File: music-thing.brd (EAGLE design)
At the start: 177.5 x 129.5 mm, 6 parts

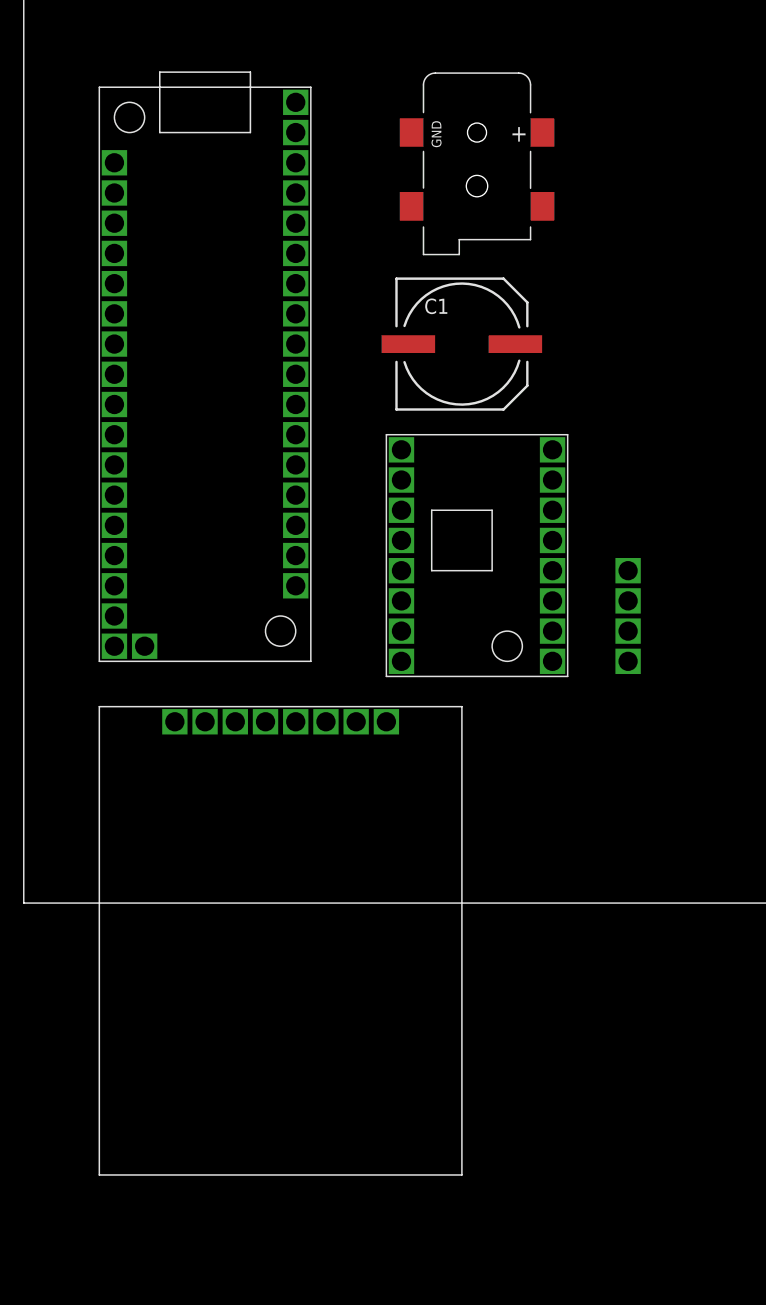
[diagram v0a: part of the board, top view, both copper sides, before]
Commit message: finalize
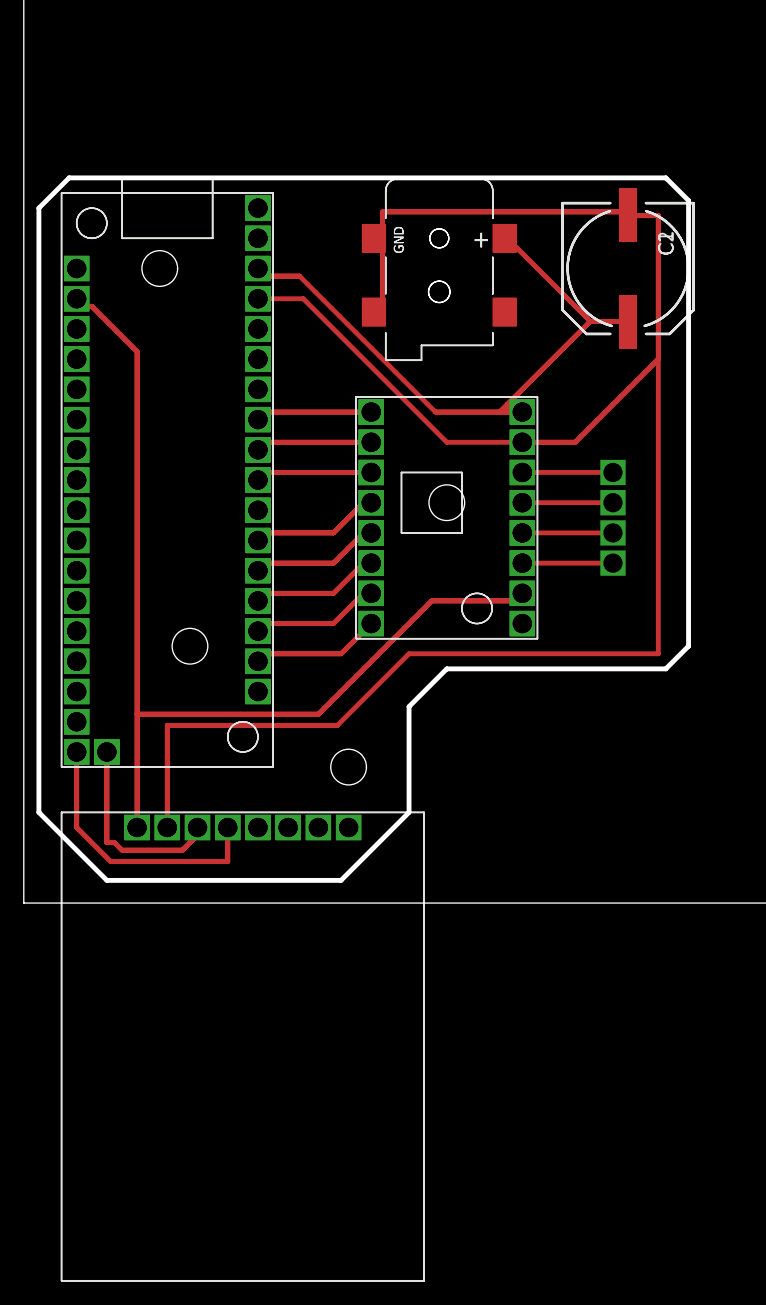
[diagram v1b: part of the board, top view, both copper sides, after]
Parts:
- added C2: 100uF, SparkFun-Capacitors:NIC_10X10.5_CAP
- added CN2: (no value), adafruit:DCJACK_2MM_SMT
- added E$1: (no value), weller-eagle:CON-MOTOR
- added U$5: ASTAR32U4MINI, weller-eagle:ASTAR32U4MINI
- added U$6: CON-USB-READER-V18, weller-eagle:CON-USB-READER-V18
- U$4: value CON-MOTOR -> A4998; device weller-eagle:CON-MOTOR -> weller-eagle:A4998
- moved U$4 20.4 mm to (27.9, 22.2)
- moved C1 15.3 mm to (50.8, 53.3), turned to 270 degrees
- moved U$2 9.44 mm to (3.17, 11.4)
- moved U$3 9.44 mm to (33.7, -31.8)
- moved CN1 9.44 mm to (34.9, 55.9)
- moved U$1 4.07 mm to (27.9, 22.2)
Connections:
- removed net N$1: U$1.2B, U$4.A1
- removed net N$2: U$1.2A, U$4.A2
- removed net N$3: U$1.1A, U$4.B1
- removed net N$4: U$1.1B, U$4.B2
- new net 5V1: U$4.VDD, U$5.5V, U$6.VCC
- new net GND1: C2.-, CN2.GND, CN2.GNDBREAK, U$4.GND1, U$6.GND1
- new net N$16: U$4.DIR, U$5.PB3
- new net N$17: U$4.STP, U$5.PB2
- new net N$18: U$4.!SLP, U$5.PB1
- new net N$19: U$4.!RST, U$5.PB0
- new net N$20: U$4.MS3, U$5.PD5
- new net N$21: U$4.MS2, U$5.PF0
- new net N$22: U$4.MS1, U$5.PF1
- new net N$23: U$4.!EN, U$5.PF4
- new net N$24: C2.+, CN2.PWR1, U$4.VMOT, U$5.VIN
- new net N$25: U$5.PE2, U$6.TX
- new net N$26: U$5.PD2, U$6.TXR
- new net S$1: U$3.GND1
- new net S$2: E$1.A1, U$1.2B
- new net S$3: E$1.A2, U$1.2A
- new net S$4: E$1.B1, U$1.1A
- new net S$5: E$1.B2, U$1.1B
- net GND: now also U$1.GND1, U$2.GND2; no longer U$3.GND1
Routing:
- net GND1: track 0.00 -> 107.0 mm
- net GND: track 0.00 -> 86.6 mm
- net 5V1: track 0.00 -> 83.5 mm
- net 5V: track 0.00 -> 83.5 mm
- net S$1: track 0.00 -> 52.3 mm
- net N$24: track 0.00 -> 52.0 mm
- net N$5: track 0.00 -> 35.8 mm
- net N$26: track 0.00 -> 23.1 mm
- net N$15: track 0.00 -> 23.1 mm
- net N$25: track 0.00 -> 16.7 mm
- net N$14: track 0.00 -> 16.7 mm
- net N$8: track 0.00 -> 10.8 mm
- net N$7: track 0.00 -> 10.8 mm
- net N$18: track 0.00 -> 10.8 mm
- net N$17: track 0.00 -> 10.8 mm
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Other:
- outline, holes or cut-outs redrawn

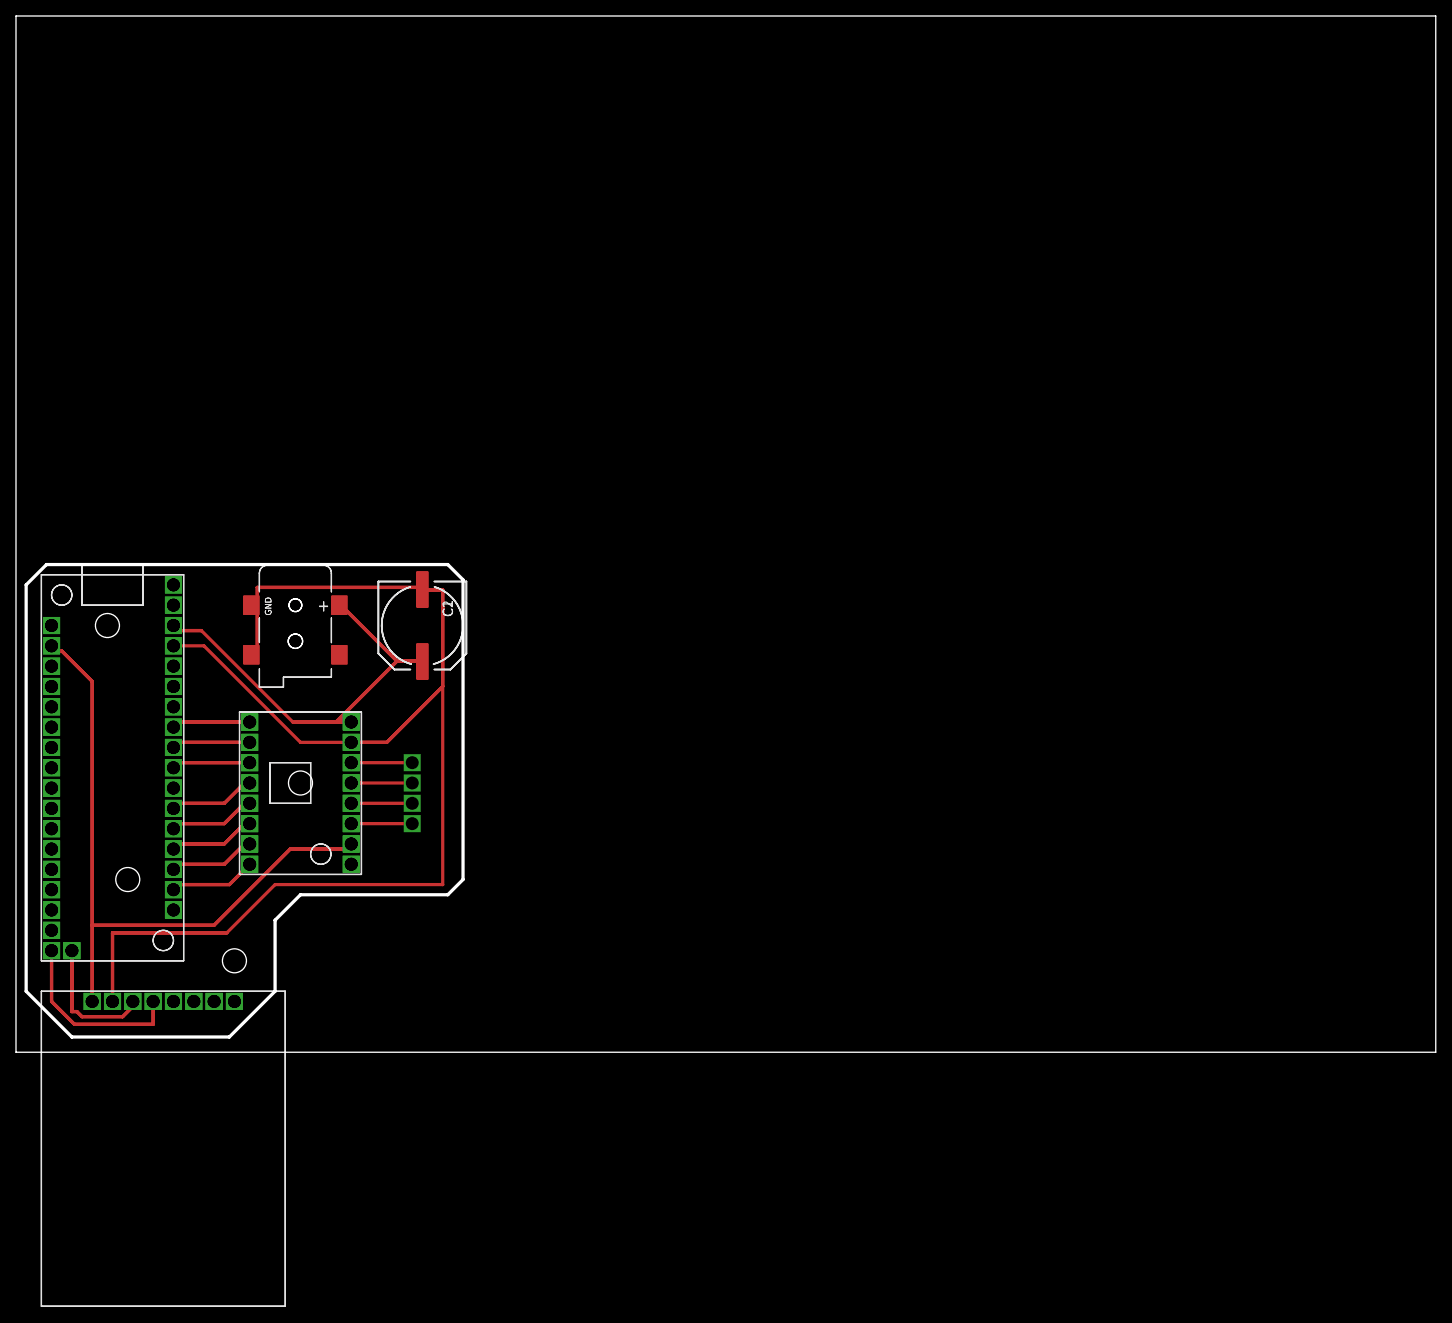
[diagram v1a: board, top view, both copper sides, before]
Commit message: new board
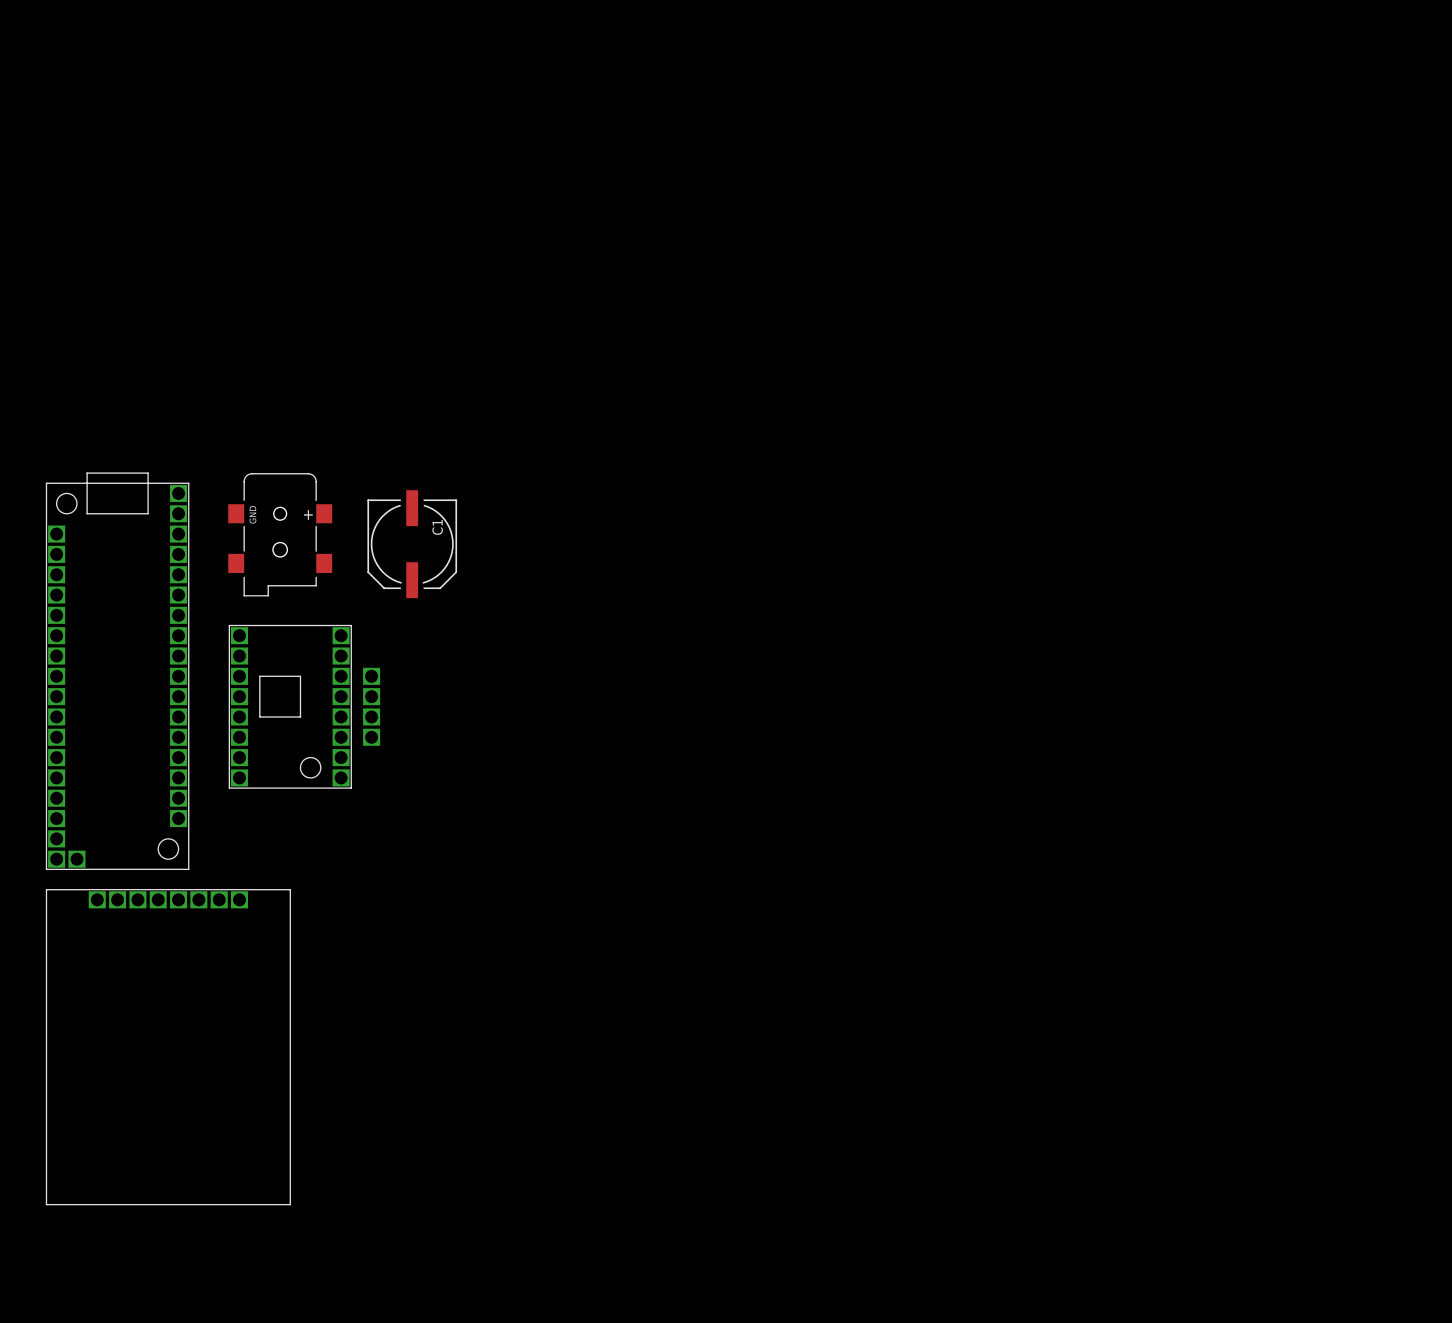
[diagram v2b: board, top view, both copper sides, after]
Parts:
- removed C2: 100uF, SparkFun-Capacitors:NIC_10X10.5_CAP
- removed CN2: (no value), adafruit:DCJACK_2MM_SMT
- removed E$1: (no value), weller-eagle:CON-MOTOR
- removed U$5: ASTAR32U4MINI, weller-eagle:ASTAR32U4MINI
- removed U$6: CON-USB-READER-V18, weller-eagle:CON-USB-READER-V18
- U$4: value A4998 -> CON-MOTOR; device weller-eagle:A4998 -> weller-eagle:CON-MOTOR
- moved U$4 22.1 mm to (41.9, 39.4)
- moved U$3 12.7 mm to (34.3, -19.1)
- moved CN1 11.6 mm to (33.0, 67.3)
- moved U$2 11.4 mm to (3.81, 22.9)
- moved U$1 10.9 mm to (26.7, 33.0)
- moved C1 10.2 mm to (49.5, 63.5)
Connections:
- removed net 5V1: U$4.VDD, U$5.5V, U$6.VCC
- removed net GND1: C2.-, CN2.GND, CN2.GNDBREAK, U$4.GND1, U$6.GND1
- removed net N$16: U$4.DIR, U$5.PB3
- removed net N$17: U$4.STP, U$5.PB2
- removed net N$18: U$4.!SLP, U$5.PB1
- removed net N$19: U$4.!RST, U$5.PB0
- removed net N$20: U$4.MS3, U$5.PD5
- removed net N$21: U$4.MS2, U$5.PF0
- removed net N$22: U$4.MS1, U$5.PF1
- removed net N$23: U$4.!EN, U$5.PF4
- removed net N$24: C2.+, CN2.PWR1, U$4.VMOT, U$5.VIN
- removed net N$25: U$5.PE2, U$6.TX
- removed net N$26: U$5.PD2, U$6.TXR
- removed net S$1: U$3.GND1
- removed net S$2: E$1.A1, U$1.2B
- removed net S$3: E$1.A2, U$1.2A
- removed net S$4: E$1.B1, U$1.1A
- removed net S$5: E$1.B2, U$1.1B
- new net N$1: U$1.2B, U$4.A1
- new net N$2: U$1.2A, U$4.A2
- new net N$3: U$1.1A, U$4.B1
- new net N$4: U$1.1B, U$4.B2
- net GND: now also U$2.GND1, U$3.GND2; no longer U$2.GND2
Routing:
- net GND1: track 107.0 -> 0.00 mm
- net GND: track 86.6 -> 0.00 mm
- net 5V1: track 83.5 -> 0.00 mm
- net 5V: track 83.5 -> 0.00 mm
- net S$1: track 52.3 -> 0.00 mm
- net N$24: track 52.0 -> 0.00 mm
- net N$5: track 35.8 -> 0.00 mm
- net N$26: track 23.1 -> 0.00 mm
- net N$15: track 23.1 -> 0.00 mm
- net N$25: track 16.7 -> 0.00 mm
- net N$14: track 16.7 -> 0.00 mm
- net N$8: track 10.8 -> 0.00 mm
- net N$7: track 10.8 -> 0.00 mm
- net N$18: track 10.8 -> 0.00 mm
- net N$17: track 10.8 -> 0.00 mm
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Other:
- board outline removed
